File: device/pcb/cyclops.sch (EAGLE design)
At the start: 180 parts, among them Q1 SSM3K324, Q2 SSM3K324, Q3 SSM3K324, Q4 IRF510, U1 MCP4921, U10 ADG1201, U11 THS4281, U12 MAX4564, U13 ZXTD, U14 ZXTD, U15 OPA1664, U2 LT1931, U3 LT1764A, U31 TPS62153, U4 BD00FC0WEFJ, U5 TPS72325, U6 LT1711, U7 TLV3701, U8 ADR03, U9 LT1880

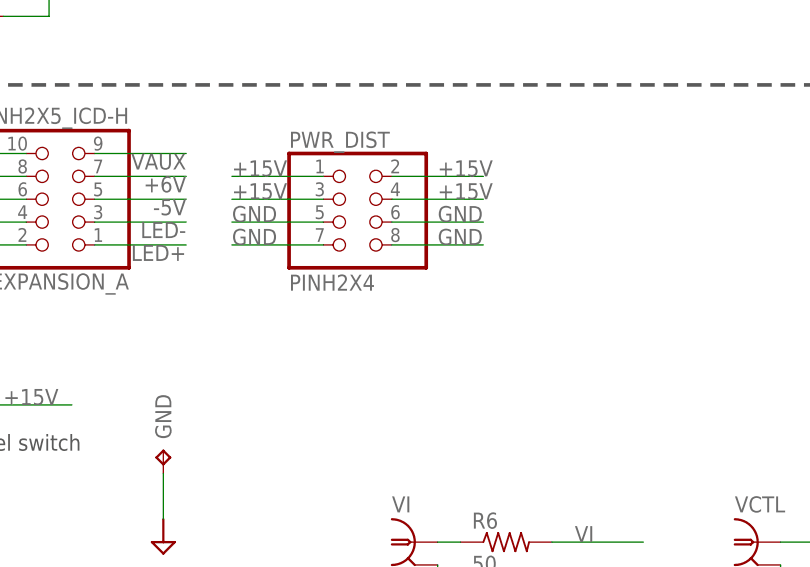
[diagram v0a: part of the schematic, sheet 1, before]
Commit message: Minor changes prior to fab of 3.6 alpha.
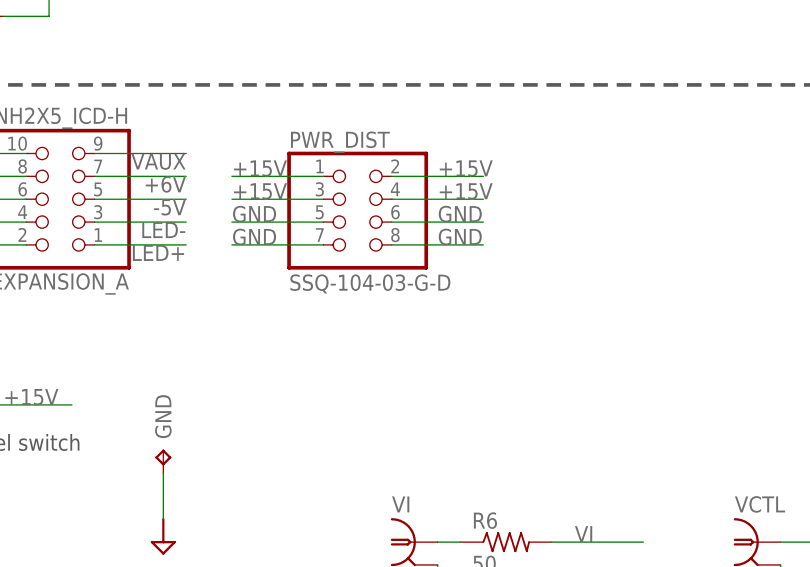
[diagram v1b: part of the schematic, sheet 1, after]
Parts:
- PWR_DIST: value PINH2X4 -> SSQ-104-03-G-D
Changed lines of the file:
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@@
 <part name="VREF" library="jonnew" deviceset="BNC" device="_0731000105" value="0731000105"/>
 <part name="VCTL" library="jonnew" deviceset="BNC" device="_0731000105" value="0731000105"/>
-<part name="PWR_DIST" library="cyclops" deviceset="PINH2X4" device=""/>
+<part name="PWR_DIST" library="cyclops" deviceset="PINH2X4" device="" value="SSQ-104-03-G-D"/>
 <part name="GAIN" library="cyclops" deviceset="POT_US" device="_3310" value="1k"/>
 <part name="VCTL&lt;OFF&gt;DAC" library="cyclops" deviceset="SPDT" device="_2M-WITHOFF" value="100-SP3"/>
